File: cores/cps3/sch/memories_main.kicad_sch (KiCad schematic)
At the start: 4 parts

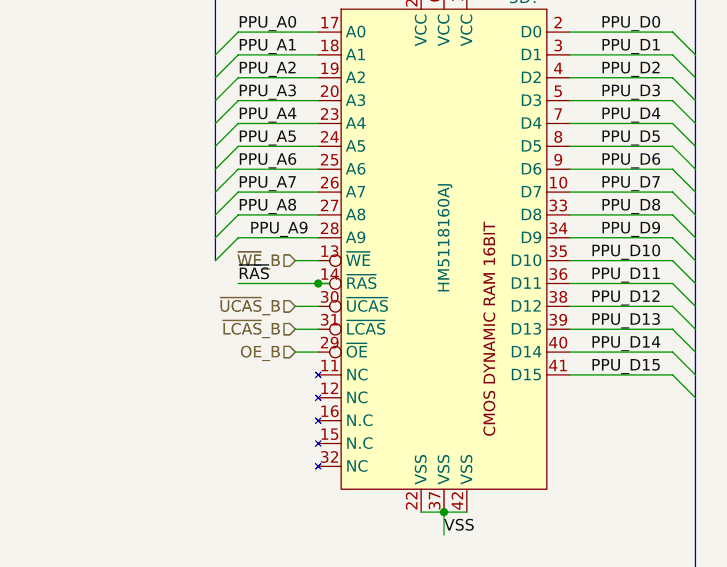
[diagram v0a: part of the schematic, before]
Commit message: update6_cps
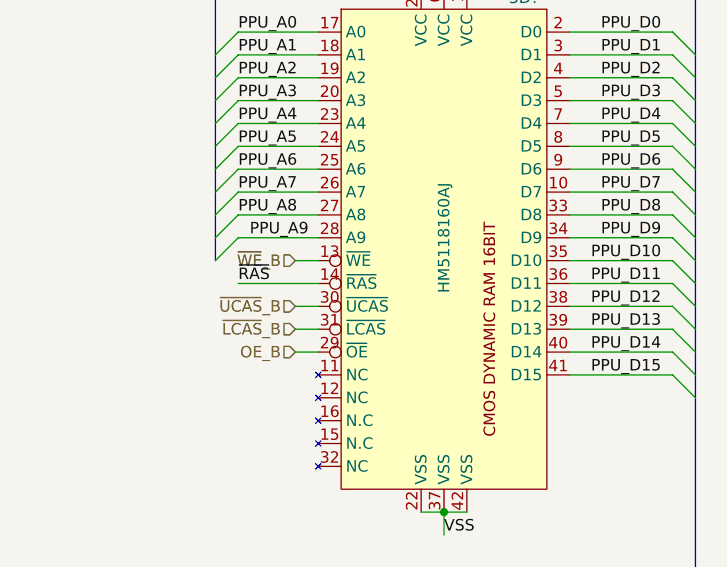
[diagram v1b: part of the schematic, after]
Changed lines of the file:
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@@
   (junction (at 74.93 30.48) (diameter 0) (color 0 0 0 0)
   )
-  (junction (at 60.96 128.27) (diameter 0) (color 0 0 0 0)
-  )
   (junction (at 154.94 97.79) (diameter 0) (color 0 0 0 0)
   )
@@
   )
   (wire (pts (xy 88.9 110.49) (xy 100.33 110.49))
-    (stroke (width 0) (type default) (color 0 0 0 0))
-  )
-  (wire (pts (xy 62.23 128.27) (xy 60.96 128.27))
     (stroke (width 0) (type default) (color 0 0 0 0))
   )
@@
       (effects (font (size 1.27 1.27)) hide)
     )
-    (property "Datasheet" "https://pdf1.alldatasheet.com/datasheet-pdf/view/122997/HITACHI/HM5118160.html" (id 3) (at 154.94 158.75 0)
+    (property "Datasheet" "https://www.ic72.com/pdf_file/h/564149.pdf" (id 3) (at 154.94 158.75 0)
       (effects (font (size 1.27 1.27)) hide)
     )
